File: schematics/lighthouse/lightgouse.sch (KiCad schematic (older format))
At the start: 12 parts, among them P1 3V3, P2 GND, U1 ESP-201, U2 rc522

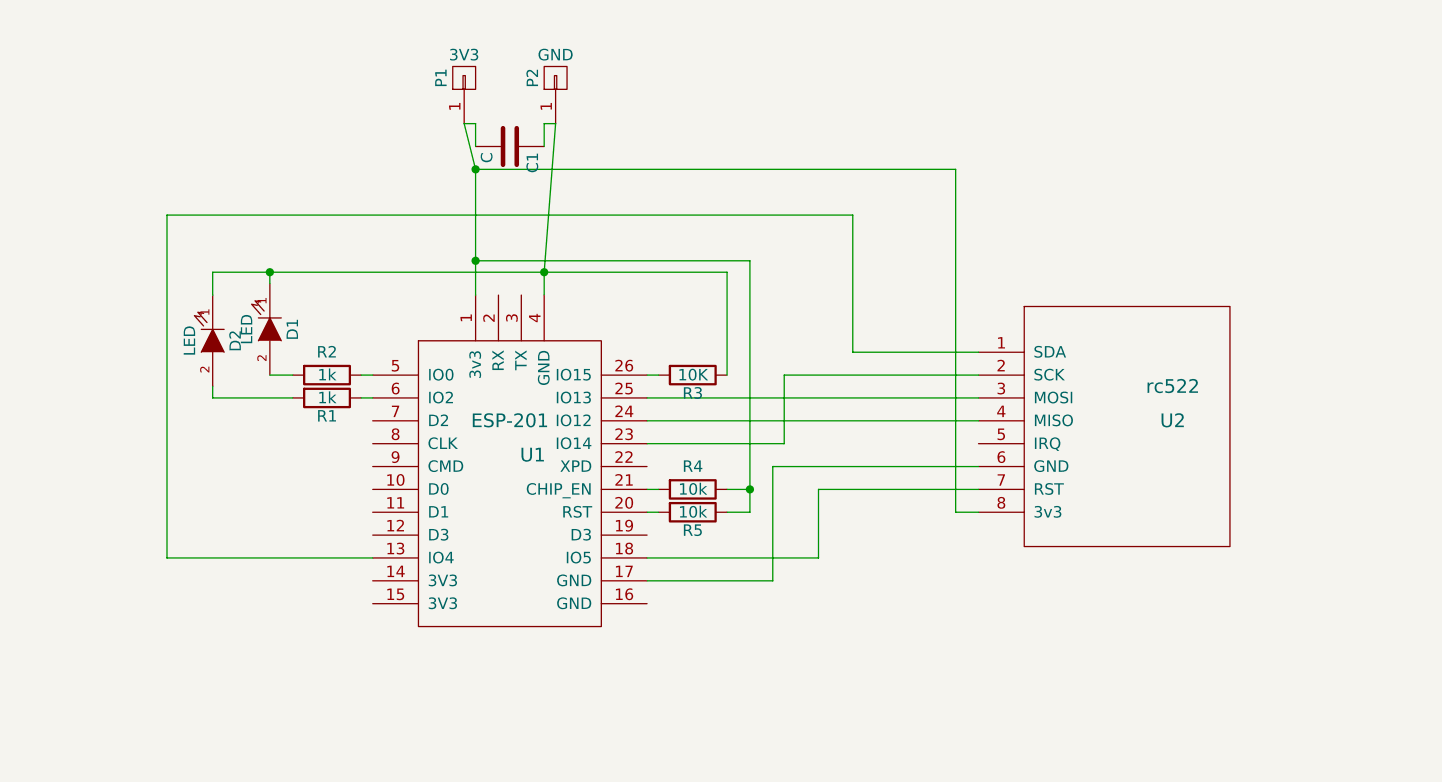
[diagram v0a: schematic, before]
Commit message: SCHEMATICS: prepare Lighthouse for production
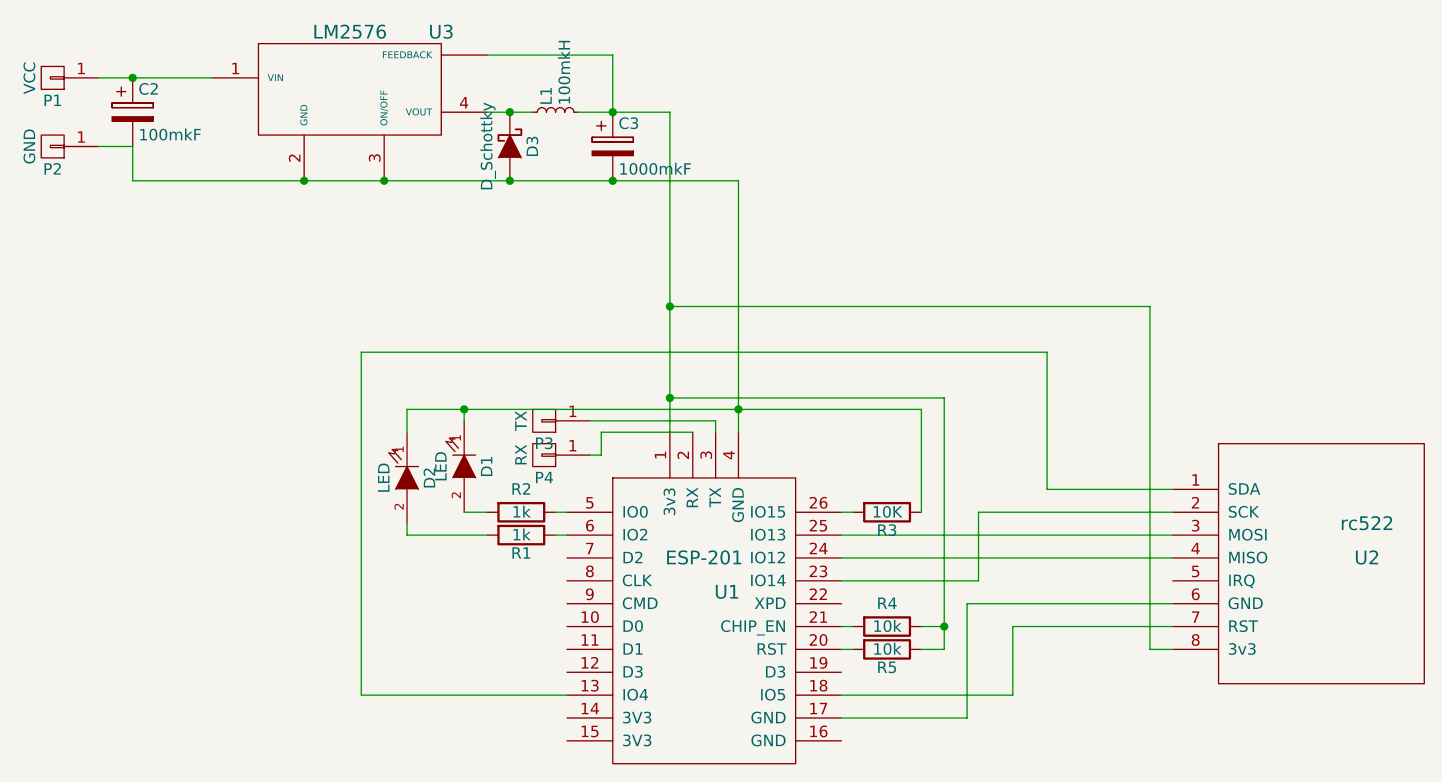
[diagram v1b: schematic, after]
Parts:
- removed C1: C, Capacitors_ThroughHole:C_Disc_D3_P2.5, symbol C
- added C2: 100mkF, bugs:capasitor, symbol CP
- added C3: 1000mkF, bugs:capasitor, symbol CP
- added D3: D_Schottky, Diodes_ThroughHole:Diode_DO-41_SOD81_Horizontal_RM10, symbol D_Schottky
- added L1: 100mkH, Discret:CP4, symbol L_Small
- added P3: TX, Pin_Headers:Pin_Header_Straight_1x01, symbol CONN_01X01
- added P4: RX, Pin_Headers:Pin_Header_Straight_1x01, symbol CONN_01X01
- added U3: LM2576, TO_SOT_Packages_THT:Pentawatt_Neutral_Straight_Vertical_TO220-5-T05A, symbol LM2576
- P1: value 3V3 -> VCC
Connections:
- net at R4.1, R5.1, U1.1 (3v3)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: now also C3.1, L1.2, U3.~ (FEEDBACK); no longer P1.1 (P1)
- net at U1.2 (RX): now also P4.1 (P1)
- net at U1.3 (TX): now also P3.1 (P1)
- net at D1.1 (K), D2.1 (K), P2.1 (P1)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: now also C2.2, C3.2, D3.2 (A), U3.2 (GND), U3.3 (ON/OFF)
- new net: C2.1, P1.1 (P1), U3.1 (VIN)
- new net: D3.1 (K), L1.1, U3.4 (VOUT)
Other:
- moved on the sheet: D1, D2, P1, P2, R1, R2, R3, R4, R5, U1, U2
